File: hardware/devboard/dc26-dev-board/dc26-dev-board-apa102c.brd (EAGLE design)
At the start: 67.3 x 91.4 mm, 84 parts, among them CN1 JST, IC1 STM32F411RET6, M10 STM32-Breakout-2, P1 SSSS811101, U1 ESP-WROOM-32, Y1 ABL-8.000MHZ-B2

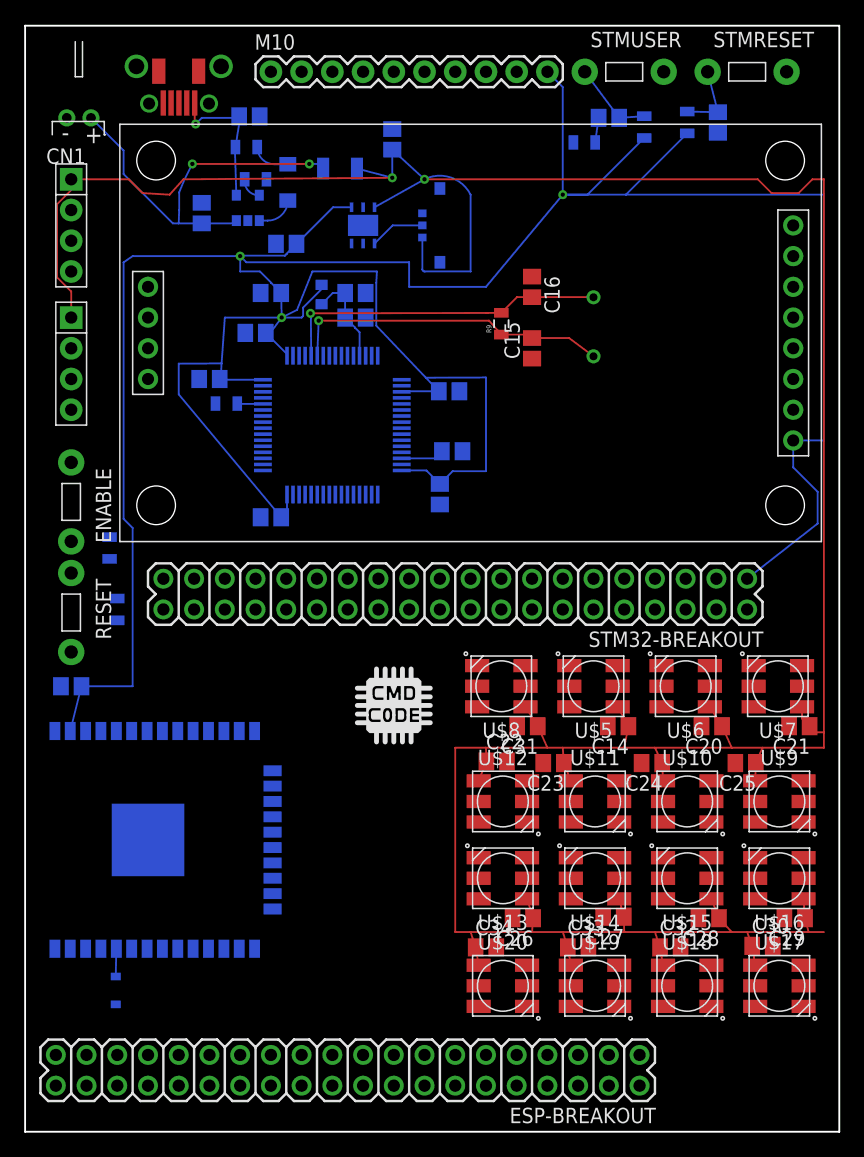
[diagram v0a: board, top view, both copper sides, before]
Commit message: board sent to oshpark
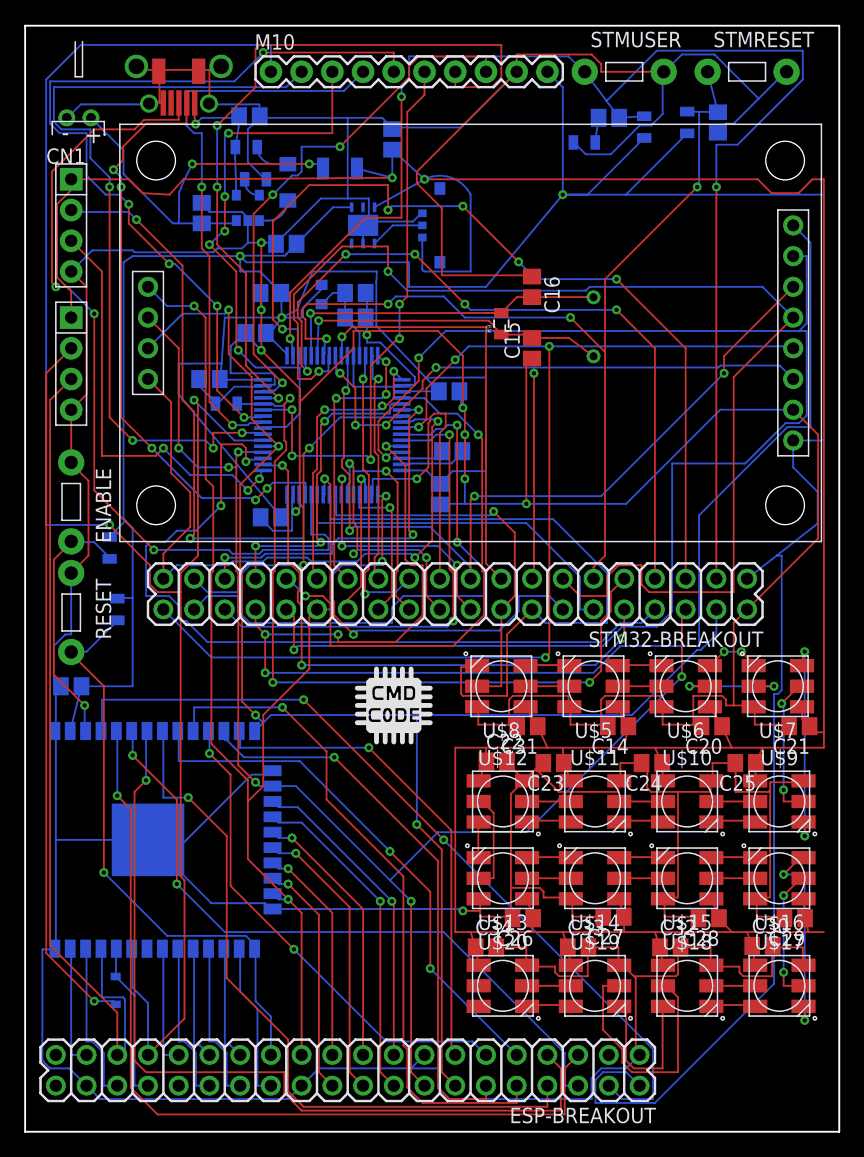
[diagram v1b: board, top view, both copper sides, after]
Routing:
- net GND: track 0.00 -> 721.8 mm, vias 0 -> 10
- net ESP_CS: track 0.00 -> 145.8 mm, vias 0 -> 2
- net SPI3_ESP_MOSI: track 0.00 -> 122.7 mm, vias 0 -> 4
- net SPI2_LCD_SCK: track 0.00 -> 120.1 mm, vias 0 -> 3
- net SPI3_ESP_MISO: track 0.00 -> 116.8 mm, vias 0 -> 6
- net LCD_BACKLIGHT: track 0.00 -> 114.3 mm, vias 0 -> 4
- net PC13: track 6.83 -> 118.2 mm, vias 0 -> 3
- net SPI3_ESP_SCK: track 0.00 -> 104.9 mm, vias 0 -> 4
- net LCD_DATA_CMD: track 0.00 -> 101.4 mm, vias 0 -> 2
- net LCD_RESET: track 0.00 -> 95.8 mm, vias 0 -> 4
- net NRST: track 5.99 -> 81.6 mm, vias 0 -> 4
- net PC14: track 0.00 -> 74.2 mm, vias 0 -> 5
- net SENSOR_VN: track 0.00 -> 72.1 mm, vias 0 -> 1
- net IO35: track 0.00 -> 70.7 mm, vias 0 -> 1
- net ESP-TX0: track 0.00 -> 70.2 mm
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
